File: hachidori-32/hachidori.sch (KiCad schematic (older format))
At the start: 45 parts, among them P1 VIN, P2 UART, P3 ADC, P4 I2C, SW1 FLASH, SW2 RESET, U1 NCP1117ST33, U2 MPU-9250, U4 BME280, U7 INA226

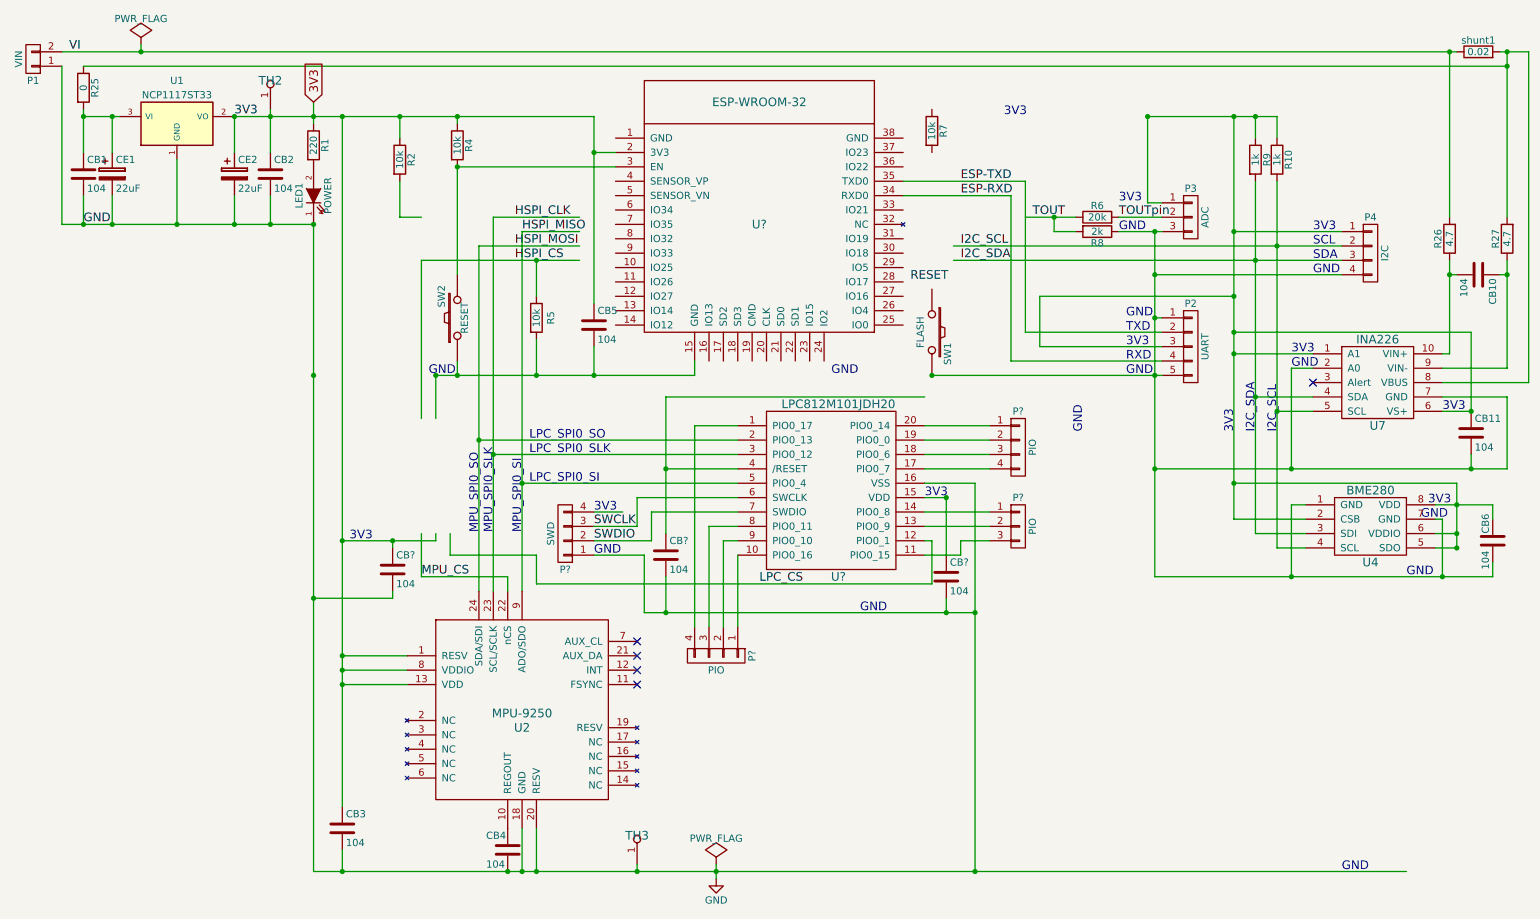
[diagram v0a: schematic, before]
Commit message: fix connections
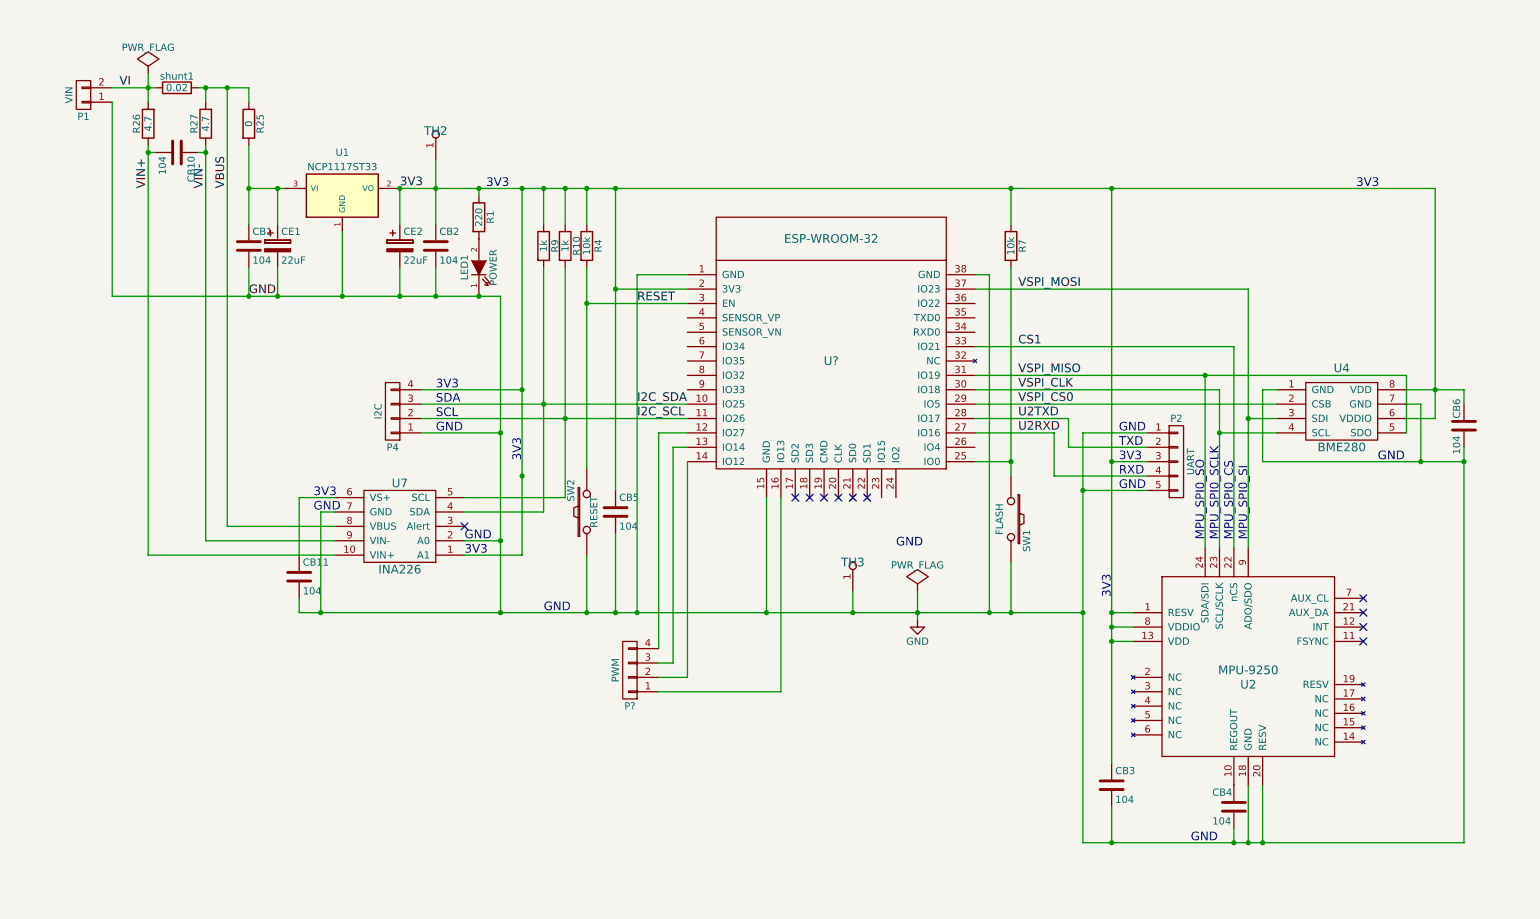
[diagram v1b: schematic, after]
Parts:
- removed CB? (x3): 104, droneworks:GRM18, symbol C
- removed P3: ADC, droneworks:Pin_Header_1x03, symbol CONN_01X03
- removed P?: SWD, symbol CONN_01X04
- removed P? (x2): PIO, symbol CONN_01X04
- removed P?: PIO, droneworks:Pin_Header_1x03, symbol CONN_01X03
- removed R2, R5: 10k, rohm:MCR03, symbol R
- removed R6: 20k, rohm:MCR03, symbol R
- removed R8: 2k, rohm:MCR03, symbol R
- removed U?: LPC812M101JDH20, symbol LPC812M101JDH20
- added P?: PWM, droneworks:Pin_Header_1x04, symbol CONN_01X04
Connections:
- net labels added: CS1, U2RXD, U2TXD, VBUS, VIN+, VIN-, VSPI_CLK, VSPI_CS0, VSPI_MISO, VSPI_MOSI
- net labels removed: ESP-RXD, ESP-TXD, HSPI_CLK, HSPI_CS, HSPI_MISO, HSPI_MOSI, LPC_CS, MPU_CS, SWCLK, SWDIO, TOUT, TOUTpin
- wire segments 171 -> 179
- no-connect marks 5 -> 11
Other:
- note added: "MPU_SPI0_CS"
- note added: "MPU_SPI0_SCLK"
- note removed: "I2C_SCL"
- note removed: "I2C_SDA"
- note removed: "LPC_SPI0_SI"
- note removed: "LPC_SPI0_SLK"
- note removed: "LPC_SPI0_SO"
- note removed: "MPU_SPI0_SLK"
- moved on the sheet: CB1, CB10, CB11, CB2, CB3, CB4, CB5, CB6, CE1, CE2, LED1, P1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
